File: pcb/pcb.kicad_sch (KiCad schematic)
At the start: 64 parts, among them J1 WH, J2 RGB, J3 220, Q1 AO3400A, Q2 AO3400A, Q3 AO3400A, Q4 AO3400A, Q5 2N60, Q6 DTD114E, Q7 AO3400A, SW1 mode, SW2 bright, T1 ., U1 ATtiny13A-SS, U2 TNY268G, U3 PC817, U4 TL431DBZ, U5 AZ1117-5.0

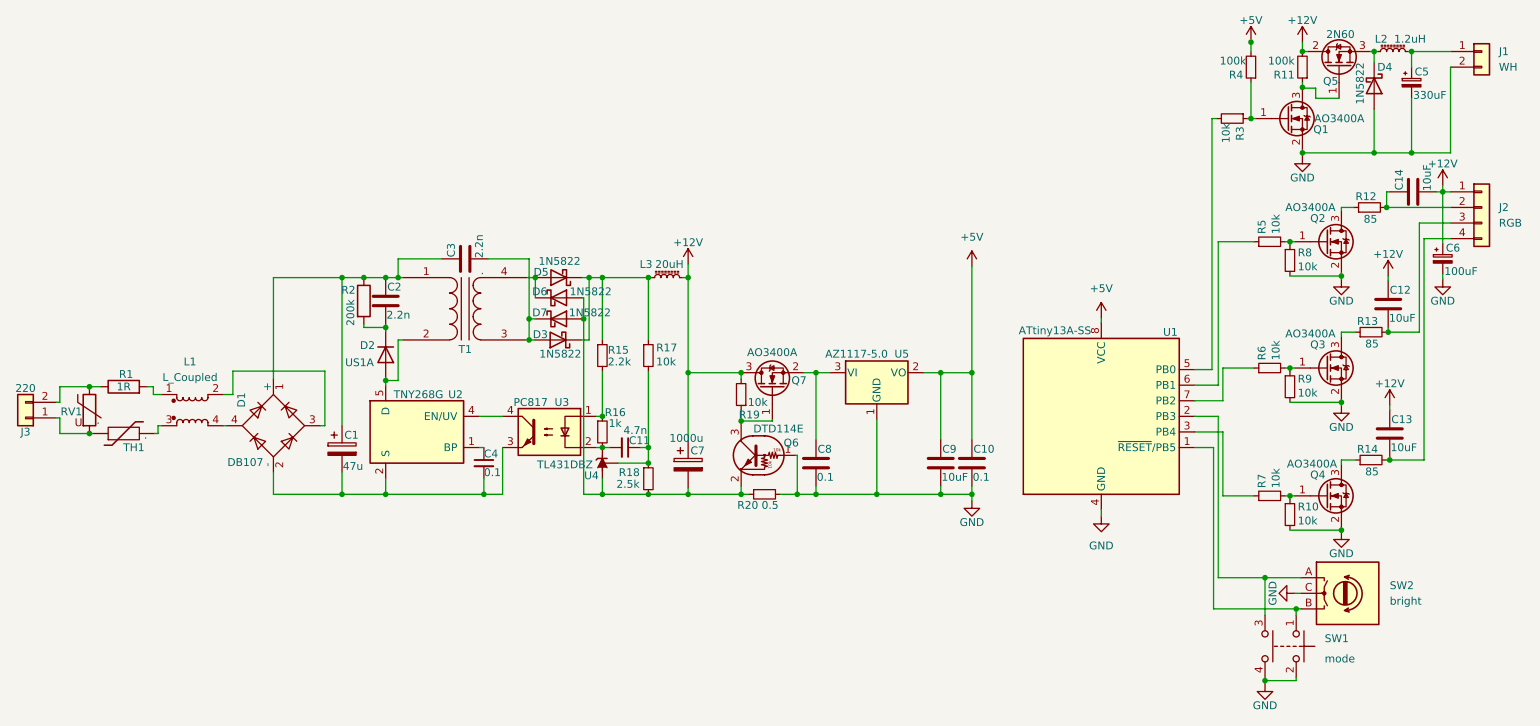
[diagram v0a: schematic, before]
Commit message: pcb ok, code is coming
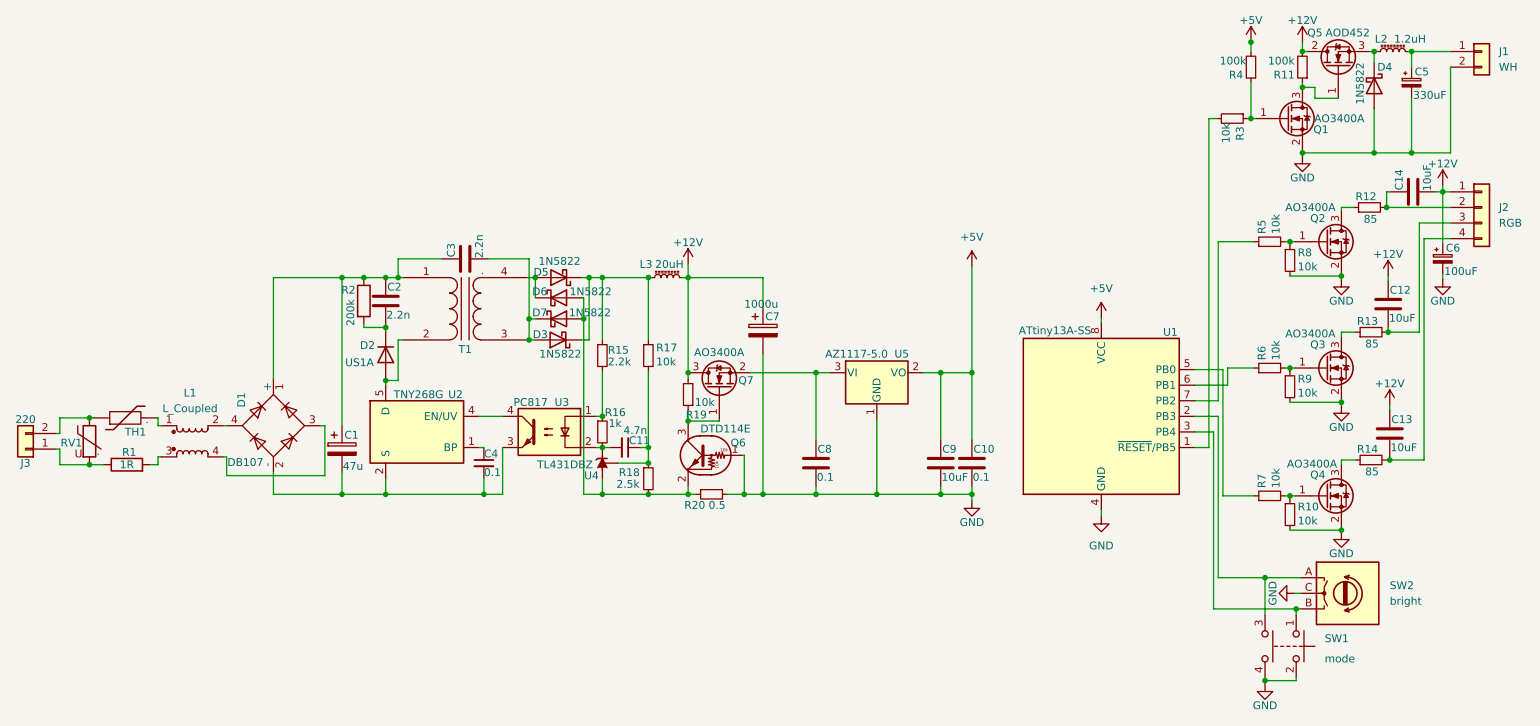
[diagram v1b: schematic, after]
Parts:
- removed Q5: 2N60, Package_TO_SOT_THT:TO-220-3_Vertical, symbol Transistor_FET:IRF740
- added Q5: AOD452, Package_TO_SOT_SMD:TO-252-2, symbol Transistor_FET:QM6006D
- C1: footprint Capacitor_THT:C_Axial_L3.8mm_D2.6mm_P7.50mm_Horizontal -> Capacitor_THT:CP_Radial_D13.0mm_P7.50mm
- C11: footprint Capacitor_SMD:C_0805_2012Metric -> Capacitor_SMD:C_0402_1005Metric
- R15: footprint Resistor_SMD:R_0805_2012Metric -> Resistor_SMD:R_0402_1005Metric
- SW1: footprint Button_Switch_THT:SW_PUSH_6mm -> local:SW_PUSH_6mm_2cont
- T1: footprint (none) -> local:Transformer_NF_ETAL_P1165
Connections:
- net +12V: now also Q5.2 (D)
- net GND: now also C7.2
- net at Q1.3 (D), R11.1: now also Q5.1 (G)
- net at D6.2 (A), D7.2 (A), Q6.2 (E)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: no longer C7.2
- net at J3.2 (Pin_2), RV1.1: now also TH1.1; no longer R1.1
- net at J3.1 (Pin_1), RV1.2: now also R1.1; no longer TH1.1
- net at D4.1 (K), L2.1: now also Q5.3 (S)
- net at SW1.1, SW2.B: now also U1.3 (PB4); no longer U1.1 (~{RESET}/PB5)
- net at R6.1: now also U1.6 (PB1); no longer U1.7 (PB2)
- net at D1.3: now also L1.4; no longer L1.2
- net at D1.4: now also L1.2; no longer L1.4
- net at TH1.2: now also L1.1; no longer L1.3
- net at R5.1: now also U1.7 (PB2); no longer U1.6 (PB1)
- net at R3.2: now also U1.1 (~{RESET}/PB5); no longer U1.5 (PB0)
- net at R7.1: now also U1.5 (PB0); no longer U1.3 (PB4)
- net at R1.2: now also L1.3; no longer L1.1
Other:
- moved on the sheet: C7, J3, L1, Q6, Q7, R1, R19, R20, RV1, TH1
